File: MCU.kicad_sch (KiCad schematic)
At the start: 15 parts, among them U5 STM32F405RGTx, Y1 LFXTAL055207Bulk

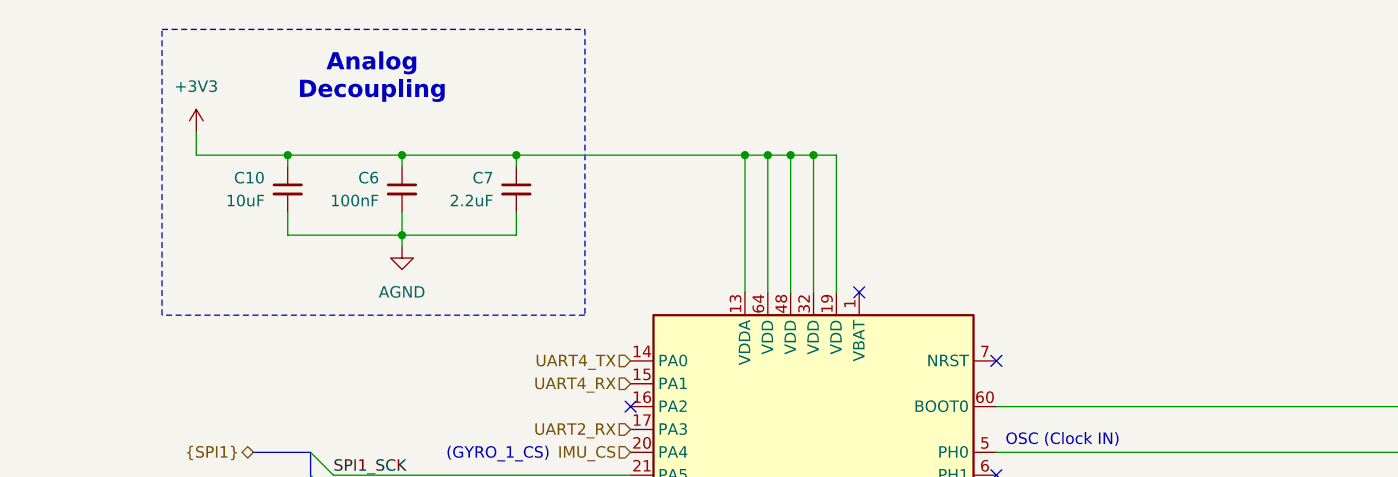
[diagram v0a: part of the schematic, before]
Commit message: Layout half-way done.
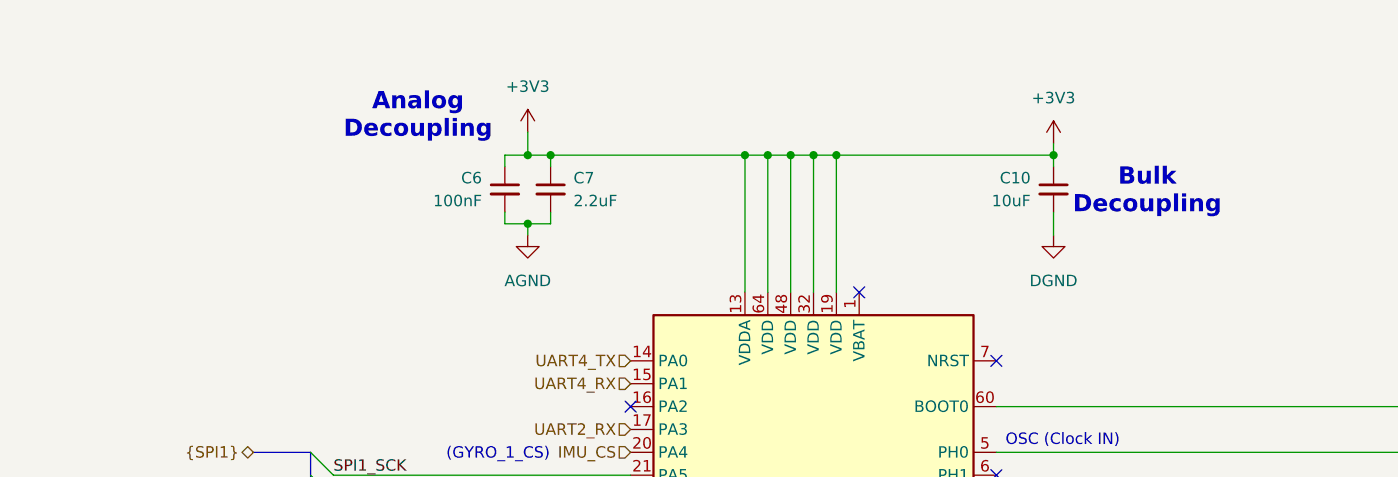
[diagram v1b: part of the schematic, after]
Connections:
- net AGND: no longer C10.2
- net DGND: now also C10.2
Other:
- note added: "Bulk Decoupling"
- moved on the sheet: C10, C6, C7
